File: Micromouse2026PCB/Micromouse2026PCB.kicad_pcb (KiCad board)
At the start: 2 copper layers, 24.9 x 25.5 mm, 15 parts, among them J1 Power Terminal, J2 i2c OLED, J3 BNO085, SW1 RotaryEncoder_Switch, U6 L7805

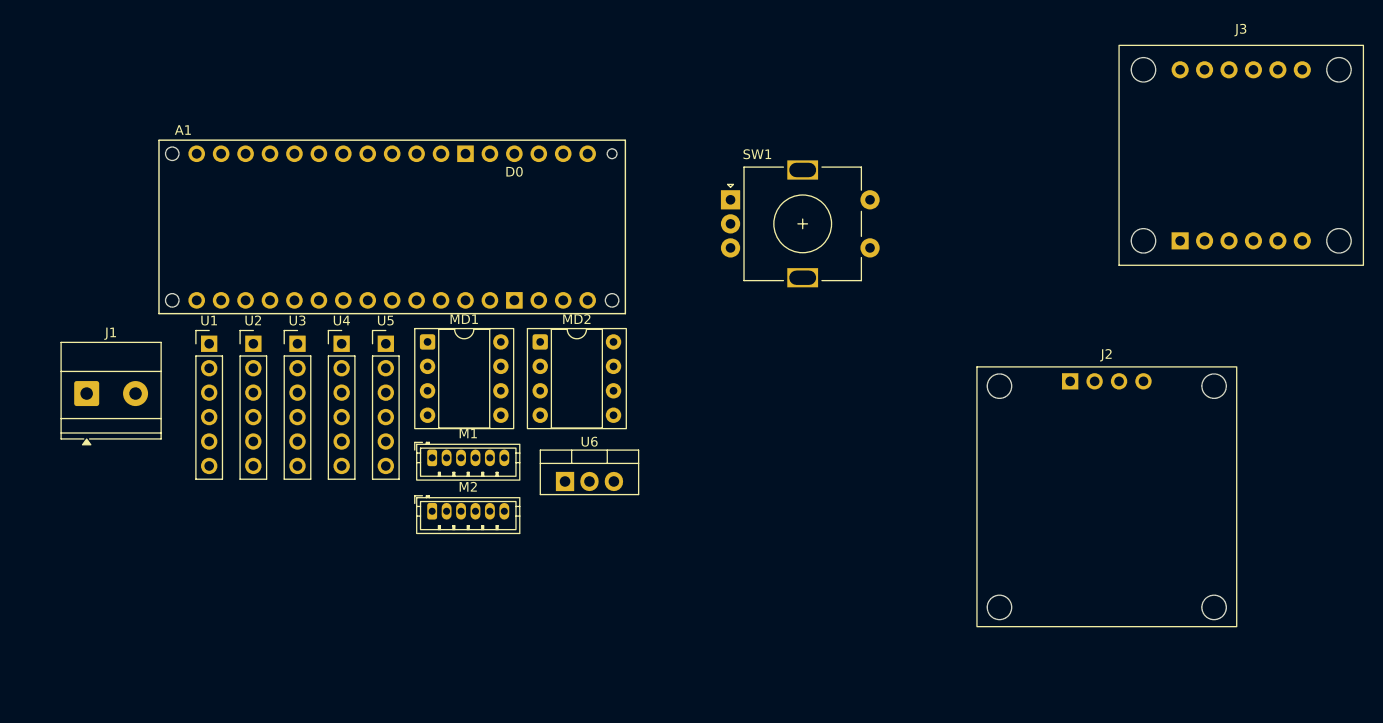
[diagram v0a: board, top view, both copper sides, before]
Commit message: PCB working version
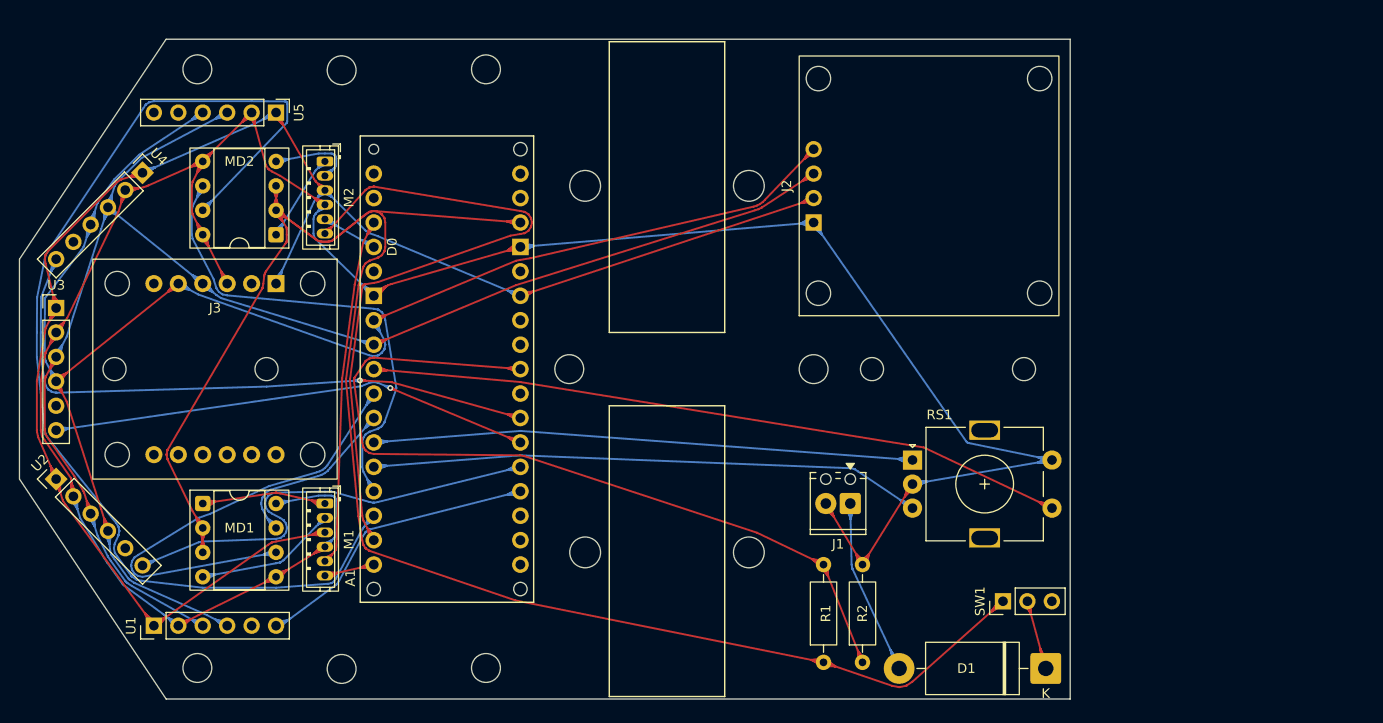
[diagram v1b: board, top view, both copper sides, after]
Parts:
- removed U6: L7805, Package_TO_SOT_THT:TO-220-3_Vertical
- added D1: 1N5822, Diode_THT:D_DO-201AD_P15.24mm_Horizontal, F.Cu at (123.2, 88.3)
- added R1: 10k, Resistor_THT:R_Axial_DIN0207_L6.3mm_D2.5mm_P10.16mm_Horizontal, F.Cu at (100.1, 87.6)
- added R2: 10k, Resistor_THT:R_Axial_DIN0207_L6.3mm_D2.5mm_P10.16mm_Horizontal, F.Cu at (104.1, 87.6)
- added SW1: PowerSW, Connector_PinHeader_2.54mm:PinHeader_1x03_P2.54mm_Vertical, F.Cu at (118.7, 81.3)
- J1: footprint TerminalBlock_Phoenix:TerminalBlock_Phoenix_MKDS-1,5-2-5.08_1x02_P5.08mm_Horizontal -> TerminalBlock_Phoenix:TerminalBlock_Phoenix_MPT-0,5-2-2.54_1x02_P2.54mm_Horizontal
- moved J3 94.1 mm to (43.2, 48.3), turned to 180 degrees
- moved J1 80.2 mm to (102.9, 71.1), turned to 180 degrees
- moved A1 49.2 mm to (70.0, 81.4), turned to 90 degrees
- moved M2 38.0 mm to (48.3, 35.6), turned to -90 degrees
- moved RS1 33.0 mm to (109.3, 66.6)
- moved J2 31.4 mm to (99.1, 41.9), turned to 90 degrees
- moved U1 29.9 mm to (30.5, 83.8), turned to 90 degrees
- moved MD2 29.6 mm to (43.2, 43.2), turned to 180 degrees
- moved MD1 28.8 mm to (35.6, 71.1)
- moved U4 27.3 mm to (29.3, 36.7), turned to -45 degrees
- moved U5 26.6 mm to (43.2, 30.5), turned to -90 degrees
- moved U3 25.4 mm to (20.3, 50.8)
- moved U2 24.9 mm to (20.3, 68.6), turned to 45 degrees
- moved M1 12.1 mm to (48.3, 71.1), turned to -90 degrees
- renumbered SW1 to RS1
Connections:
- A1 pad A4: Net-(M1-OB) -> unconnected-(A1-PadA4)
- A1 pad A5: Net-(M2-OB) -> Net-(A1-PadA5)
- A1 pad D11: unconnected-(A1-PadD11) -> Net-(M2-OB)
- A1 pad D12: unconnected-(A1-PadD12) -> Net-(M1-OB)
- A1 pad VIN: Net-(J1-Pin_1) -> Net-(SW1-Pin_1)
- J1 pad 1: Net-(J1-Pin_1) -> Net-(D1-A)
- MD1 pad 2: Net-(U6-OUT) -> Net-(SW1-Pin_1)
- MD1 pad 3: Net-(U6-OUT) -> Net-(SW1-Pin_1)
- MD2 pad 2: Net-(U6-OUT) -> Net-(SW1-Pin_1)
- MD2 pad 3: Net-(U6-OUT) -> Net-(SW1-Pin_1)
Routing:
- net GND: track 0.00 -> 513.9 mm
- net +5V: track 0.00 -> 313.3 mm
- net Net-(SW1-Pin_1): track 0.00 -> 271.6 mm
- net /SDA: track 0.00 -> 255.9 mm
- net /SCL: track 0.00 -> 243.8 mm
- net Net-(MD2-IB): track 0.00 -> 127.7 mm
- net Net-(A1-PadA5): track 0.00 -> 112.7 mm
- net Net-(A1-PadD4): track 0.00 -> 88.3 mm
- net Net-(M2-OB): track 0.00 -> 82.6 mm
- net Net-(U4-XSHUT): track 0.00 -> 79.7 mm, vias 0 -> 1
- net Net-(A1-PadD8): track 0.00 -> 73.1 mm
- net Net-(A1-D7_INT4): track 0.00 -> 69.8 mm
- net Net-(U3-XSHUT): track 0.00 -> 66.0 mm, vias 0 -> 1
- net Net-(MD2-IA): track 0.00 -> 62.9 mm
- net Net-(MD1-IA): track 0.00 -> 61.3 mm
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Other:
- board size 24.9 x 25.5 mm -> 109.2 x 68.6 mm
